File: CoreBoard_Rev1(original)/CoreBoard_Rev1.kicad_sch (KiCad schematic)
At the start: 86 parts, among them J1 RJ45_LED_Shielded, SW1 SW_Push, SW10 SW_Push, SW11 SW_Push, SW12 SW_Push, SW13 SW_Push, SW14 SW_Push, SW15 SW_Push, SW16 SW_SPDT, SW2 SW_Push, SW3 SW_Push, SW4 SW_Push, SW5 SW_Push, SW6 SW_Push, SW7 SW_Push, SW8 SW_Push, SW9 SW_Push, U1 Teensy4.1_DEV-16771, U2 TSR_1-2450, U4 74HC148, U5 74HC148, U6 74HC00, U7 OKI

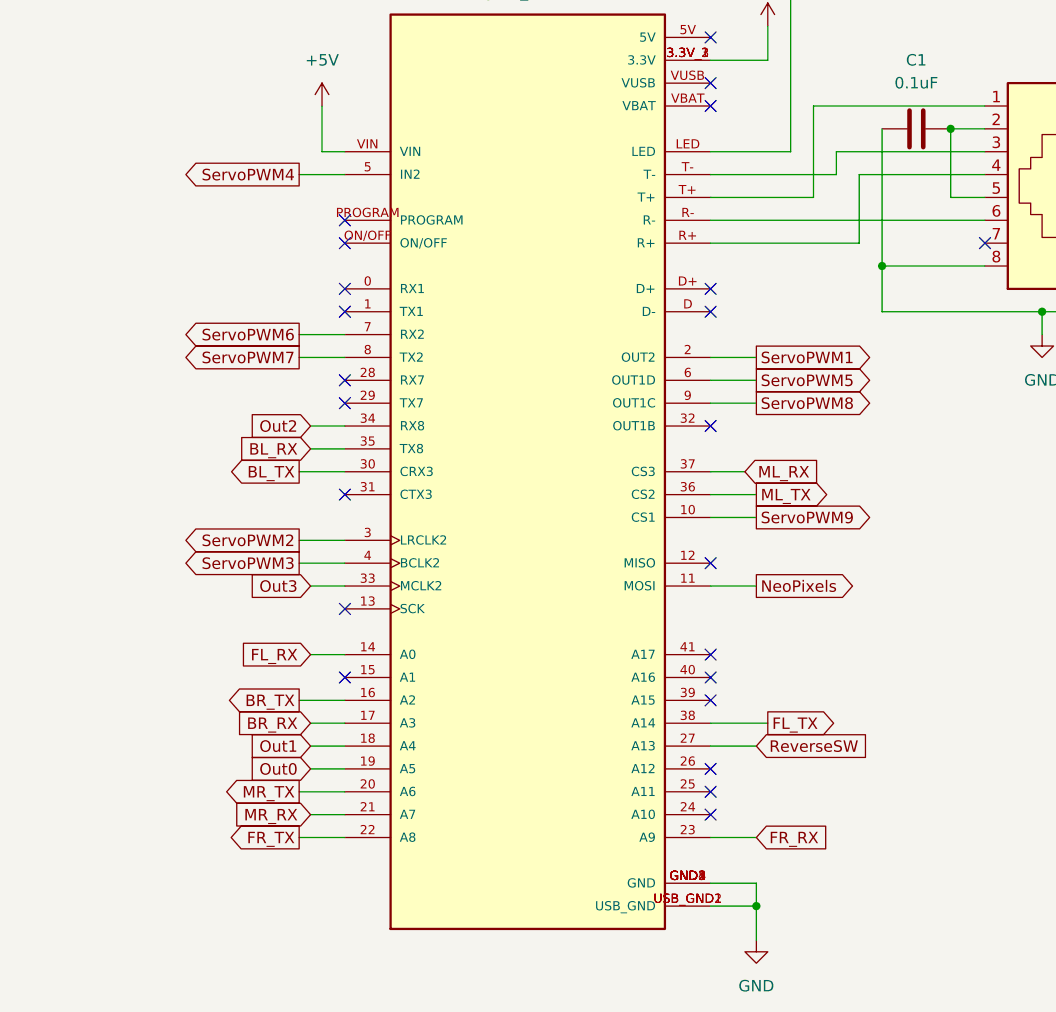
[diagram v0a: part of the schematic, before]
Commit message: re-did board
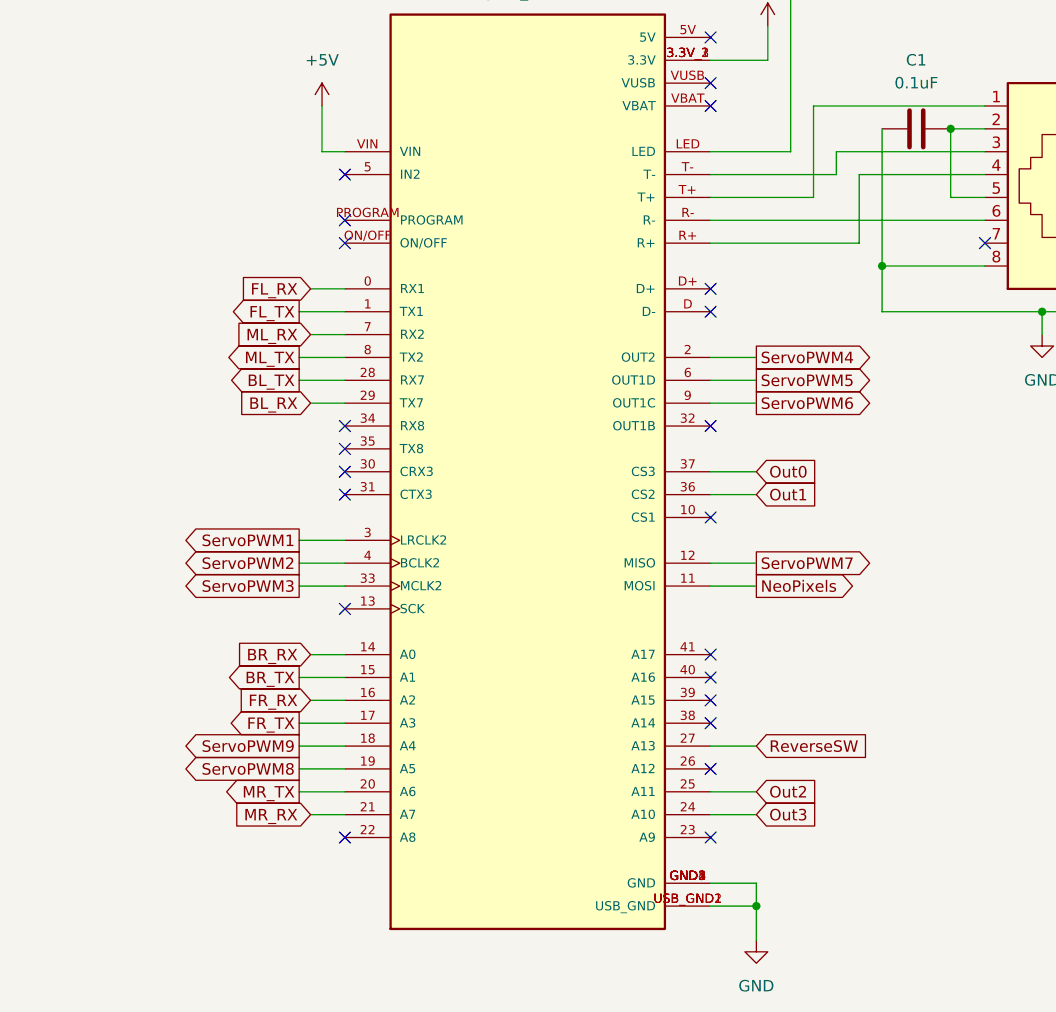
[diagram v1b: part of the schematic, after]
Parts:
- Conn2, Conn3, Conn4, Conn5, Conn6: footprint MRDT_Connectors:MOLEX_SL_09_Horizontal -> MRDT_Connectors:MOLEX_SL_09_Vertical
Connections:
- net BL_RX: now also U1.29 (TX7); no longer U1.35 (TX8)
- net BL_TX: now also U1.28 (RX7); no longer U1.30 (CRX3)
- net BR_RX: now also U1.14 (A0); no longer U1.17 (A3)
- net BR_TX: now also U1.15 (A1); no longer U1.16 (A2)
- net FL_RX: now also U1.0 (RX1); no longer U1.14 (A0)
- net FL_TX: now also U1.1 (TX1); no longer U1.38 (A14)
- net FR_RX: now also U1.16 (A2); no longer U1.23 (A9)
- net FR_TX: now also U1.17 (A3); no longer U1.22 (A8)
- net ML_RX: now also U1.7 (RX2); no longer U1.37 (CS3)
- net ML_TX: now also U1.8 (TX2); no longer U1.36 (CS2)
- net Out0: now also U1.37 (CS3); no longer U1.19 (A5)
- net Out1: now also U1.36 (CS2); no longer U1.18 (A4)
- net Out2: now also U1.25 (A11); no longer U1.34 (RX8)
- net Out3: now also U1.24 (A10); no longer U1.33 (MCLK2)
- net ServoPWM1: now also U1.3 (LRCLK2); no longer U1.2 (OUT2)
- net ServoPWM2: now also U1.4 (BCLK2); no longer U1.3 (LRCLK2)
- net ServoPWM3: now also U1.33 (MCLK2); no longer U1.4 (BCLK2)
- net ServoPWM4: now also U1.2 (OUT2); no longer U1.5 (IN2)
- net ServoPWM6: now also U1.9 (OUT1C); no longer U1.7 (RX2)
- net ServoPWM7: now also U1.12 (MISO); no longer U1.8 (TX2)
- net ServoPWM8: now also U1.19 (A5); no longer U1.9 (OUT1C)
- net ServoPWM9: now also U1.18 (A4); no longer U1.10 (CS1)
